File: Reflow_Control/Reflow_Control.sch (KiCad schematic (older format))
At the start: 62 parts

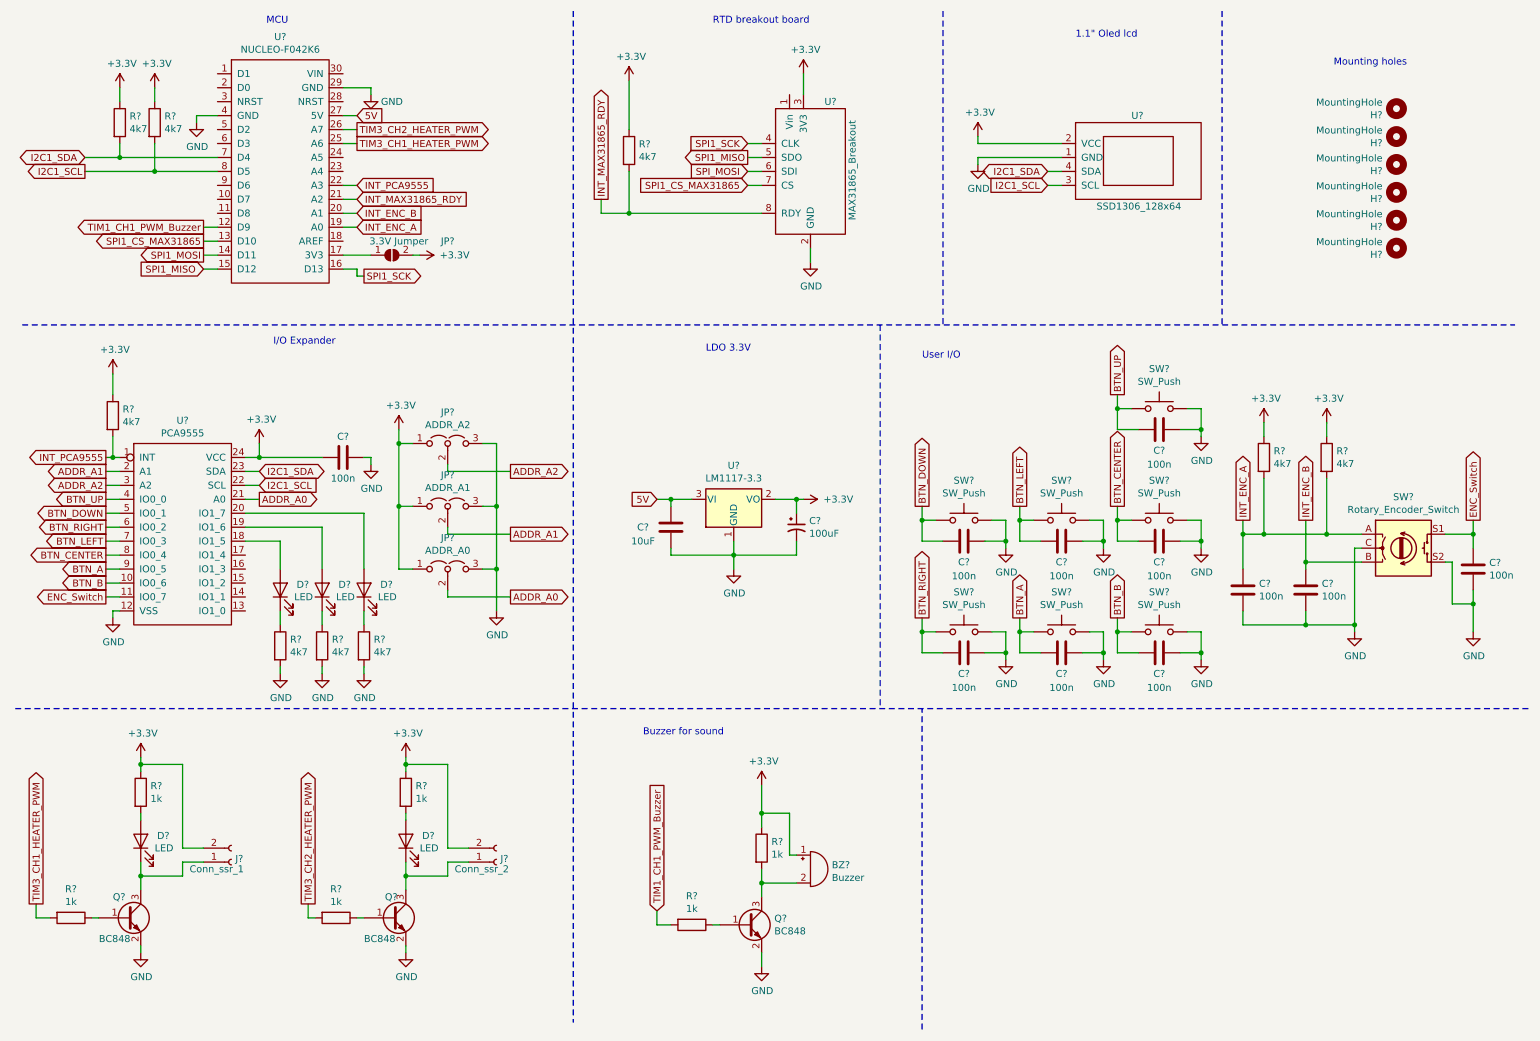
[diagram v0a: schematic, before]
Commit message: work on scematic
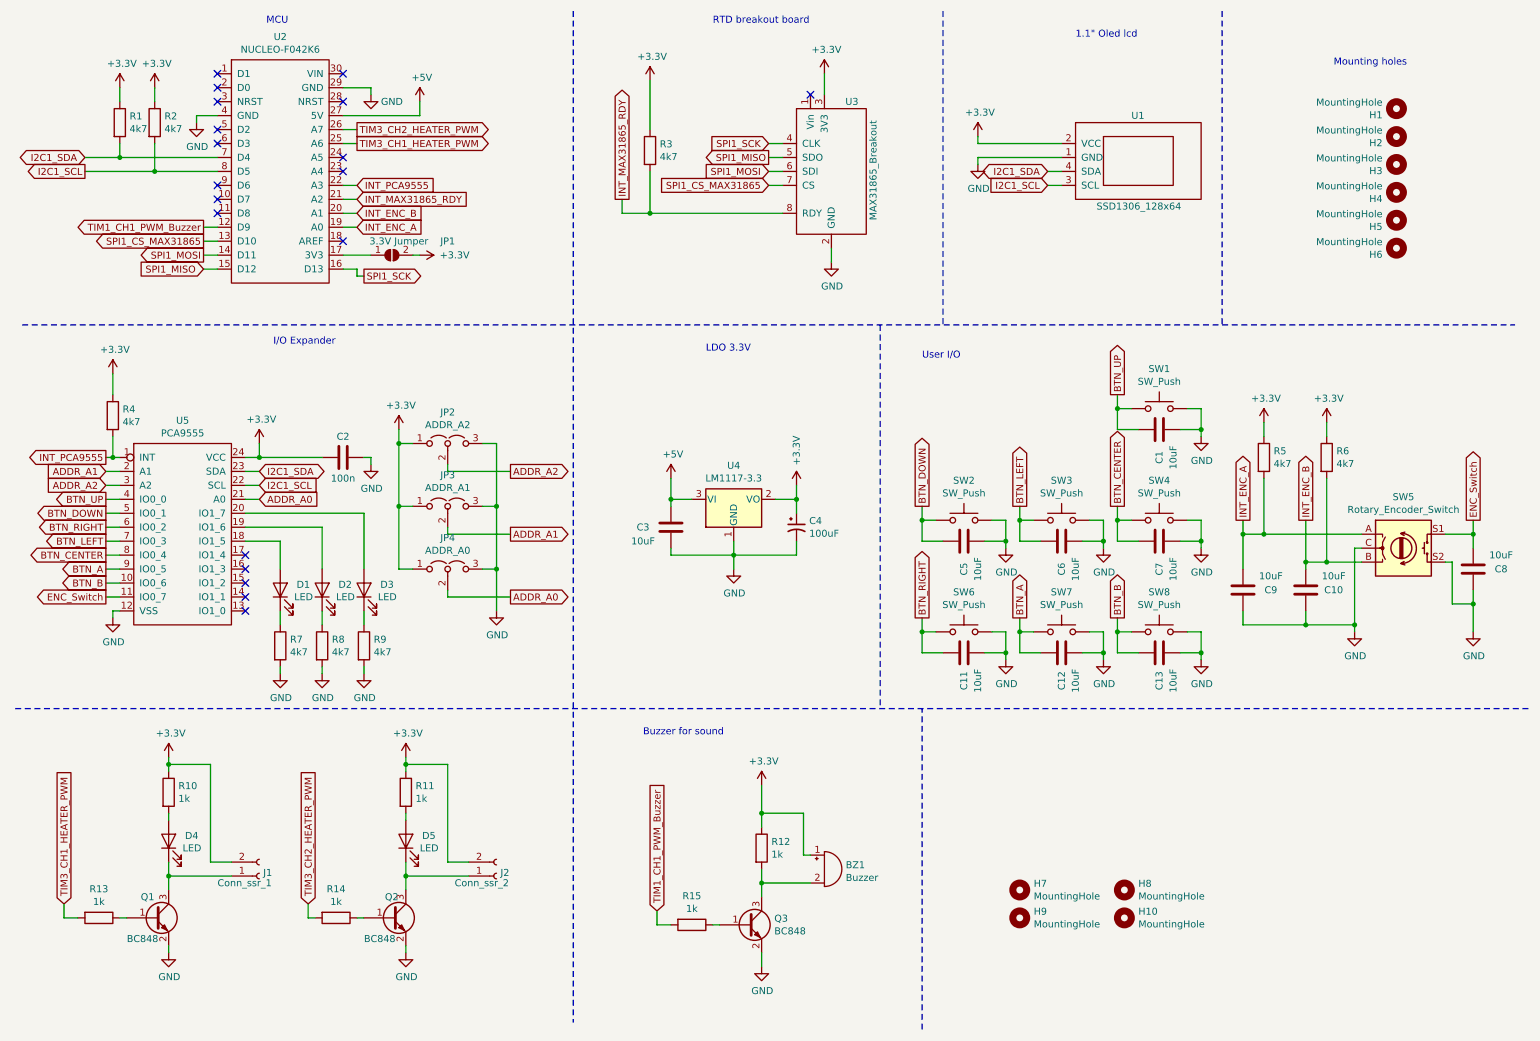
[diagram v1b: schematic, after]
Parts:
- removed C? (x10): 100n, Capacitor_SMD:C_0805_2012Metric_Pad1.15x1.40mm_HandSolder, symbol Device:C
- added C1, C10, C11, C12, C13, C5, C6, C7, C8, C9: 10uF, Capacitor_SMD:C_0805_2012Metric_Pad1.15x1.40mm_HandSolder, symbol Device:C
- added H10, H7, H8, H9: MountingHole, MountingHole:MountingHole_3mm_Pad_Via, symbol Mechanical:MountingHole
- U4: renamed from U?; footprint (none) -> Package_TO_SOT_SMD:SOT-223
- gave numbers to parts that had none: 51
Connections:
- net SPI_MOSI is gone; now on net SPI1_MOSI: U3.6 (SDI)
- net BTN_A: now also C12.1
- net BTN_B: now also C13.1
- net BTN_CENTER: now also C7.1
- net BTN_DOWN: now also C5.1
- net BTN_LEFT: now also C6.1
- net BTN_RIGHT: now also C11.1
- net BTN_UP: now also C1.1
- net ENC_Switch: now also C8.2
- net GND: now also C1.2, C10.1, C11.2, C12.2, C13.2, C5.2, C6.2, C7.2, C8.1, C9.1
- net INT_ENC_A: now also C9.2; no longer R6.2
- net INT_ENC_B: now also R6.2, C10.2
- net 5V renamed +5V
- no-connect marks 0 -> 19
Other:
- moved on the sheet: BZ1, D4, J1, J2, Q1, R10, R13, R3, U3
